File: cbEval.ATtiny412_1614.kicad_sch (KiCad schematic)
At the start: 50 parts, among them J1 Bergstik-II_3, J10 Socket.Hor.2x5.6-5535512-4, J11 Bergstik-II_3, J12 Bergstik-II_3, J13 Bergstik-II_6, J14 Bergstik-II_6, J15 Bergstik-II_6, J16 Bergstik-II_3, J17 Bergstik-II_6, J18 Bergstik-II_3, J19 Bergstik-II_6, J2 Bergstik-II_6, J20 Bergstik-II_3, J21 Bergstik-II_3, J22 Bergstik-II_2, J23 Bergstik-II_2, J3 Keystone.4918, J4 Keystone.4918, J5 Keystone.3571, J6 Keystone.3571, J7 Socket.Hor.2x5.6-5535512-4, J8 Header.Hor.2x5.9-103326-0-05, J9 Header.Hor.2x5.9-103326-0-05, U1 ATtiny412-SSFR, U2 ATtiny1614-SSFR

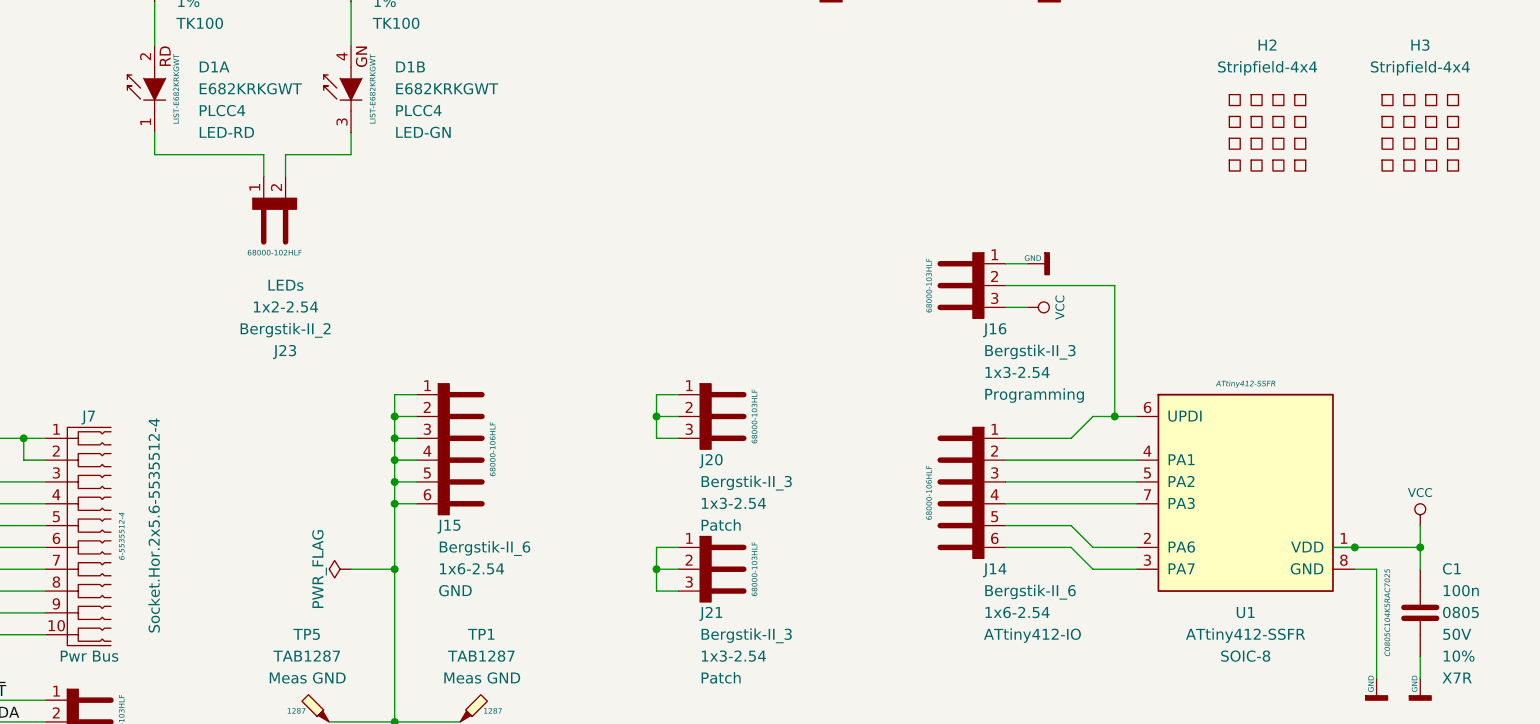
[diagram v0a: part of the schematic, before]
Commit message: kleinere Änderungen
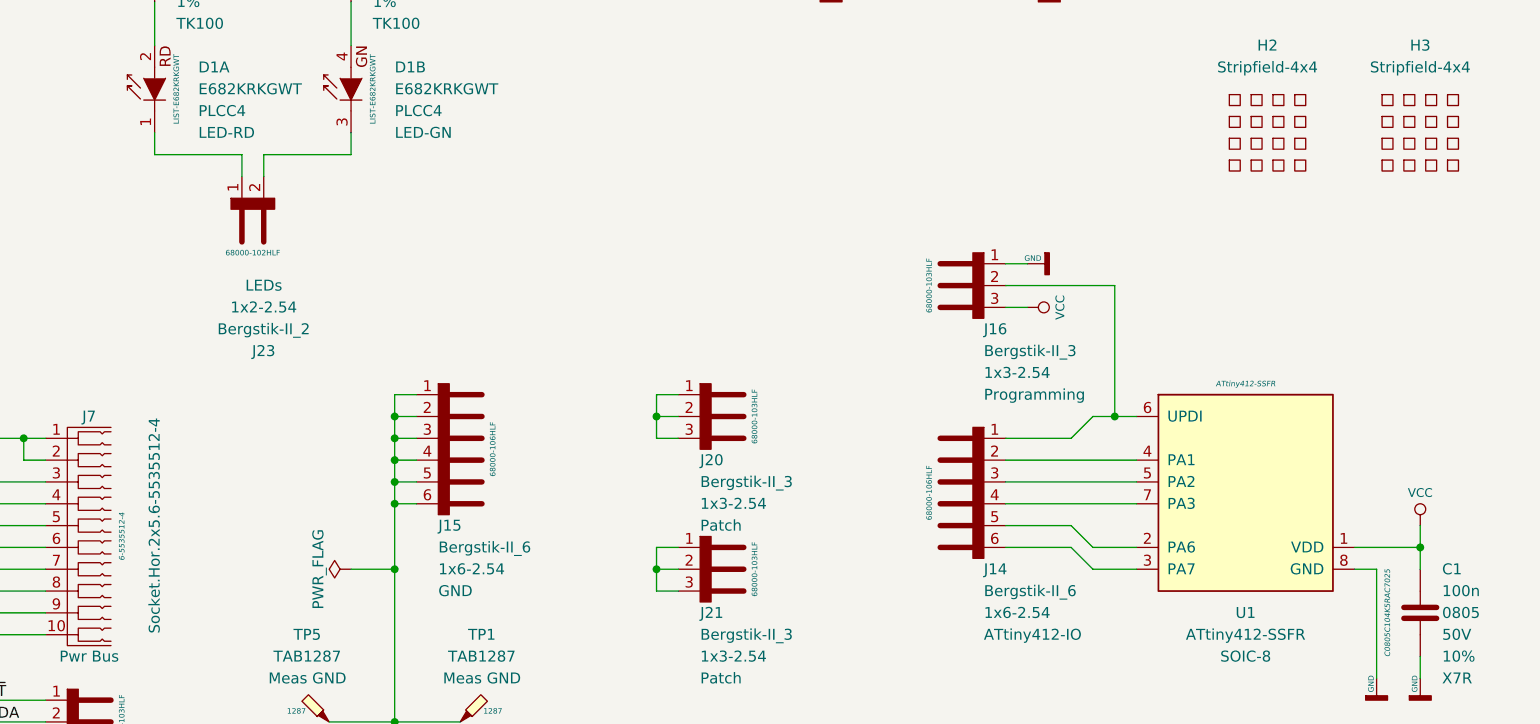
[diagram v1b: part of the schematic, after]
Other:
- moved on the sheet: J23
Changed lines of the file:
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@@
   (junction (at 238.76 129.54) (diameter 0.9144) (color 0 0 0 0))
   (junction (at 251.46 50.8) (diameter 0.9144) (color 0 0 0 0))
-  (junction (at 266.7 144.78) (diameter 0.9144) (color 0 0 0 0))
   (junction (at 274.32 144.78) (diameter 0.9144) (color 0 0 0 0))
   (no_connect (at 68.58 17.78))
@@
     (stroke (width 0) (type solid) (color 0 0 0 0))
   )
+  (wire (pts (xy 137.16 99.06) (xy 127 99.06))
+    (stroke (width 0) (type solid) (color 0 0 0 0))
+  )
+  (wire (pts (xy 137.16 101.6) (xy 137.16 99.06))
+    (stroke (width 0) (type solid) (color 0 0 0 0))
+  )
   (wire (pts (xy 139.7 35.56) (xy 139.7 38.1))
     (stroke (width 0) (type solid) (color 0 0 0 0))
@@
     (stroke (width 0) (type solid) (color 0 0 0 0))
   )
-  (wire (pts (xy 139.7 99.06) (xy 127 99.06))
+  (wire (pts (xy 139.7 99.06) (xy 149.86 99.06))
     (stroke (width 0) (type solid) (color 0 0 0 0))
   )
@@
     (stroke (width 0) (type solid) (color 0 0 0 0))
   )
-  (wire (pts (xy 142.24 99.06) (xy 149.86 99.06))
-    (stroke (width 0) (type solid) (color 0 0 0 0))
-  )
-  (wire (pts (xy 142.24 101.6) (xy 142.24 99.06))
-    (stroke (width 0) (type solid) (color 0 0 0 0))
-  )
   (wire (pts (xy 147.32 165.1) (xy 154.94 165.1))
     (stroke (width 0) (type solid) (color 0 0 0 0))
@@
     (stroke (width 0) (type solid) (color 0 0 0 0))
   )
-  (wire (pts (xy 264.16 144.78) (xy 266.7 144.78))
-    (stroke (width 0) (type solid) (color 0 0 0 0))
-  )
   (wire (pts (xy 266.7 144.78) (xy 274.32 144.78))
     (stroke (width 0) (type solid) (color 0 0 0 0))
@@
     (stroke (width 0) (type solid) (color 0 0 0 0))
   )
-  (wire (pts (xy 274.32 147.32) (xy 274.32 144.78))
+  (wire (pts (xy 274.32 144.78) (xy 274.32 147.32))
     (stroke (width 0) (type solid) (color 0 0 0 0))
   )
@@
     (pin "2")
   )
-  (symbol (lib_id "J.PinHeader:Bergstik-II_2") (at 142.24 106.68 90) (mirror x) (unit 1)
-    (in_bom yes) (on_board yes)
-    (property "Reference" "J23" (id 0) (at 142.24 121.92 90))
-    (property "Value" "Bergstik-II_2" (id 1) (at 142.24 119.38 90))
-    (property "Footprint" "Connector_PinHeader_2.54mm:PinHeader_1x02_P2.54mm_Vertical" (id 2) (at 139.7 114.3 90)
-      (effects (font (size 1.27 1.27)) hide)
-    )
-    (property "Datasheet" "https://cdn.amphenol-icc.com/media/wysiwyg/files/drawing/68000.pdf?__cf_chl_jschl_tk__=264da0a199af1bdefb04026963ad3c85a073036f-1615910483-0-AaX8LtgG8apEDzGIqgzQ0aoAKWkj50oj4JyeD-4a-BjpVTotUkz0b9CwK48SctxW9RfQ29uHK-g8U4Q7W950UfkLI47M2h-zbxXP0QVGLOROToQCZGWcFC-c_QilEUacZTRKDvvL4FAsQqyycsf3m4Eg-isf3_QP12ONd_wWQcMNK-LuQ3eyU0ZB_uGz-1tHBPJYyv3B6ZQ-xQw3v8oWI_eE_zzEWbIWrLFoFf6eZXoAoT5Y4wJiyDXoV-vBmq5F4mSG8H7EqnWkU4EpxDA2-swokem-Q60MTknd4E9RK0nSmJU_PhEDac0Sb3Im75HD1QHXcTu1yMJzQCNpgpofH-wmgz79VfPk4ttpW38ZPDdPIxv_B7gR4gWWdhvgQyW6byYqLE8E5a8tpA31lZkCN19ufDO8SqP6UAFJscCeeydKEgOe2Ksu_LJQubib6v3-6A" (id 3) (at 139.7 116.84 90)
-      (effects (font (size 1.27 1.27)) hide)
-    )
-    (property "Package" "1x2-2.54" (id 4) (at 142.24 116.84 90))
-    (property "Usage" "LEDs" (id 5) (at 142.24 114.3 90))
-    (property "ID" "68000-102HLF" (id 6) (at 140.97 110.49 90)
-      (effects (font (size 0.635 0.635)))
-    )
+  (symbol (lib_id "J.PinHeader:Bergstik-II_2") (at 139.7 106.68 90) (mirror x) (unit 1)
+    (in_bom yes) (on_board yes)
+    (property "Reference" "J23" (id 0) (at 139.7 121.92 90))
+    (property "Value" "Bergstik-II_2" (id 1) (at 139.7 119.38 90))
+    (property "Footprint" "Connector_PinHeader_2.54mm:PinHeader_1x02_P2.54mm_Vertical" (id 2) (at 137.16 114.3 90)
+      (effects (font (size 1.27 1.27)) hide)
+    )
+    (property "Datasheet" "https://cdn.amphenol-icc.com/media/wysiwyg/files/drawing/68000.pdf?__cf_chl_jschl_tk__=264da0a199af1bdefb04026963ad3c85a073036f-1615910483-0-AaX8LtgG8apEDzGIqgzQ0aoAKWkj50oj4JyeD-4a-BjpVTotUkz0b9CwK48SctxW9RfQ29uHK-g8U4Q7W950UfkLI47M2h-zbxXP0QVGLOROToQCZGWcFC-c_QilEUacZTRKDvvL4FAsQqyycsf3m4Eg-isf3_QP12ONd_wWQcMNK-LuQ3eyU0ZB_uGz-1tHBPJYyv3B6ZQ-xQw3v8oWI_eE_zzEWbIWrLFoFf6eZXoAoT5Y4wJiyDXoV-vBmq5F4mSG8H7EqnWkU4EpxDA2-swokem-Q60MTknd4E9RK0nSmJU_PhEDac0Sb3Im75HD1QHXcTu1yMJzQCNpgpofH-wmgz79VfPk4ttpW38ZPDdPIxv_B7gR4gWWdhvgQyW6byYqLE8E5a8tpA31lZkCN19ufDO8SqP6UAFJscCeeydKEgOe2Ksu_LJQubib6v3-6A" (id 3) (at 137.16 116.84 90)
+      (effects (font (size 1.27 1.27)) hide)
+    )
+    (property "Package" "1x2-2.54" (id 4) (at 139.7 116.84 90))
+    (property "Usage" "LEDs" (id 5) (at 139.7 114.3 90))
+    (property "ID" "68000-102HLF" (id 6) (at 138.43 110.49 90)
+      (effects (font (size 0.635 0.635)))
+    )

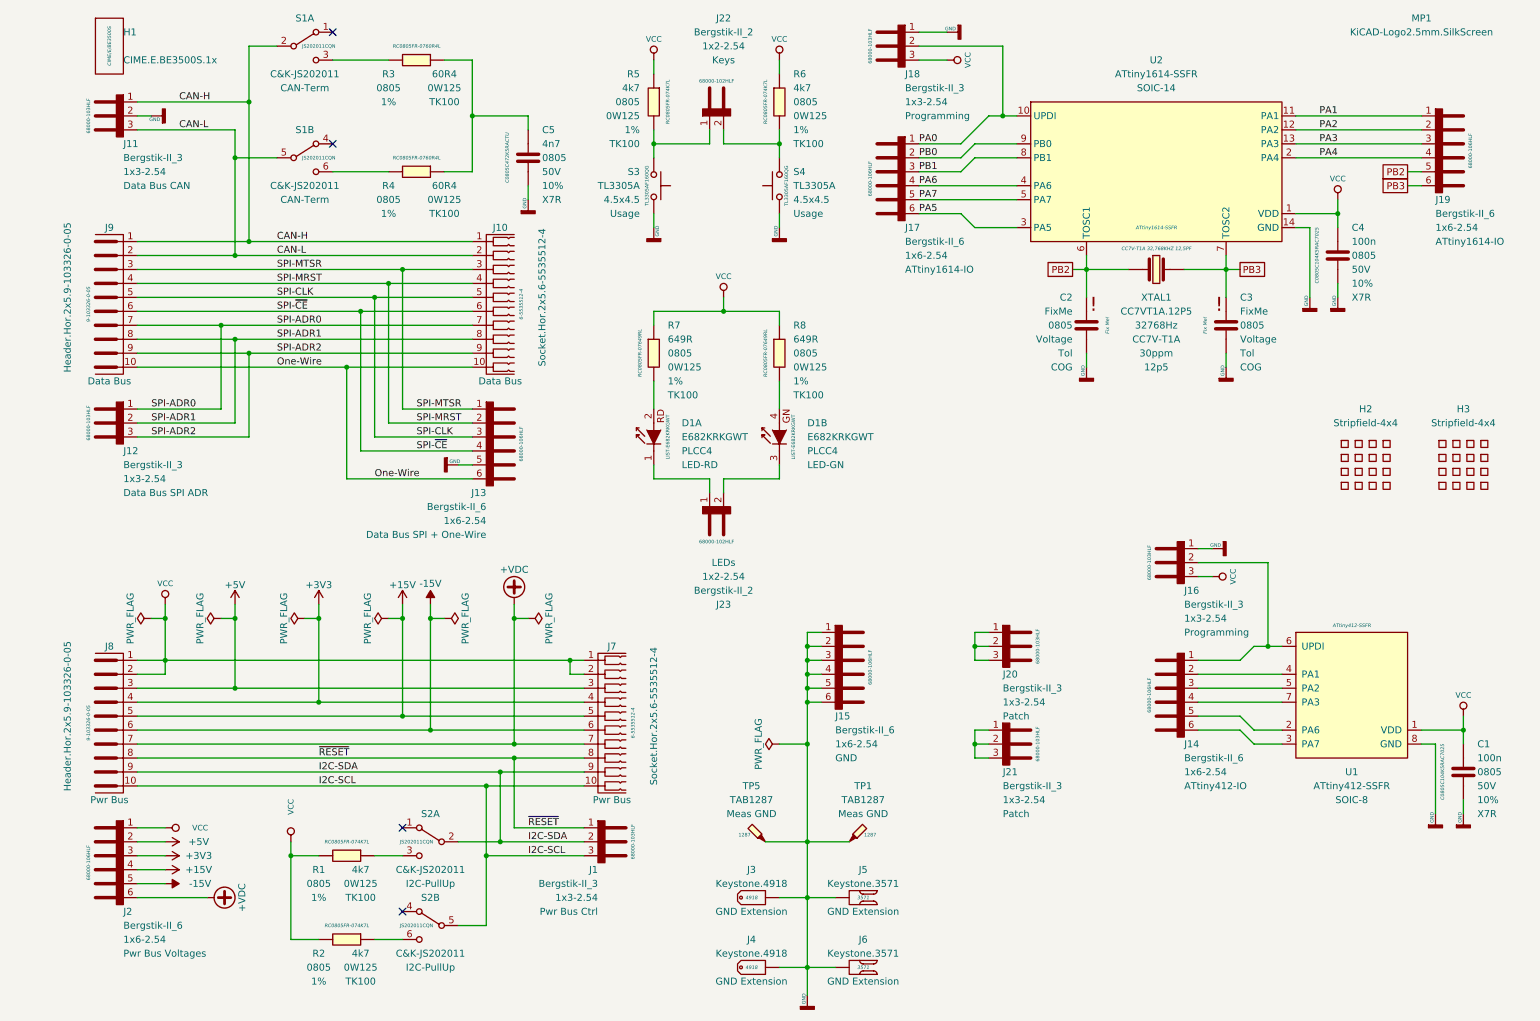
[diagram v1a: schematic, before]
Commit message: BOM erstellt und kleinere Korrekturen
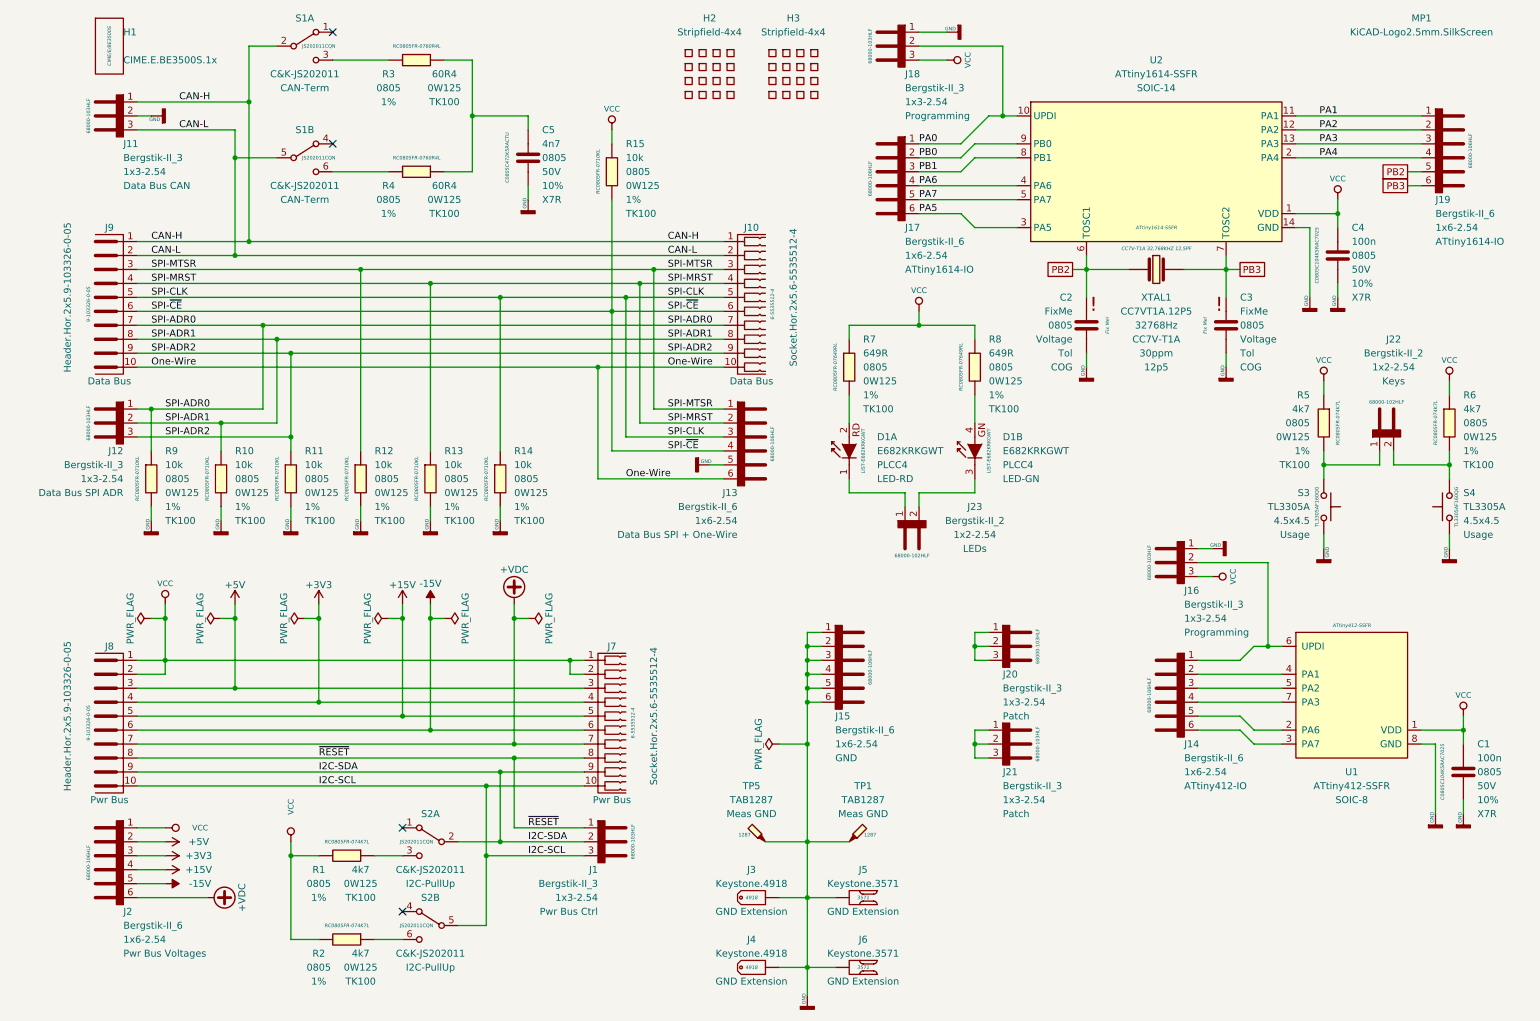
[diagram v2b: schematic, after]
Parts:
- added R10, R11, R12, R13, R14, R15, R9: 10k, Resistor_SMD:R_0805_2012Metric, symbol R.Yageo.RC0805:10k
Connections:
- net GND: now also R10.2, R11.2, R12.2, R13.2, R14.2, R9.2
- net SPI-ADR0: now also R9.1
- net SPI-ADR1: now also R10.1
- net SPI-ADR2: now also R11.1
- net SPI-CLK: now also R14.1
- net SPI-MRST: now also R13.1
- net SPI-MTSR: now also R12.1
- net SPI-~CE: now also R15.2
- net VCC: now also R15.1
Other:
- moved on the sheet: D1A, D1B, H2, H3, J10, J13, J22, J23, R5, R6, R7, R8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
